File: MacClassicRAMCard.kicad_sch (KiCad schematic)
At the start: 22 parts, among them J1 RAM Exp., U1 AS4C1M16F5, U2 AS4C1M16F5, U3 74HCT08D

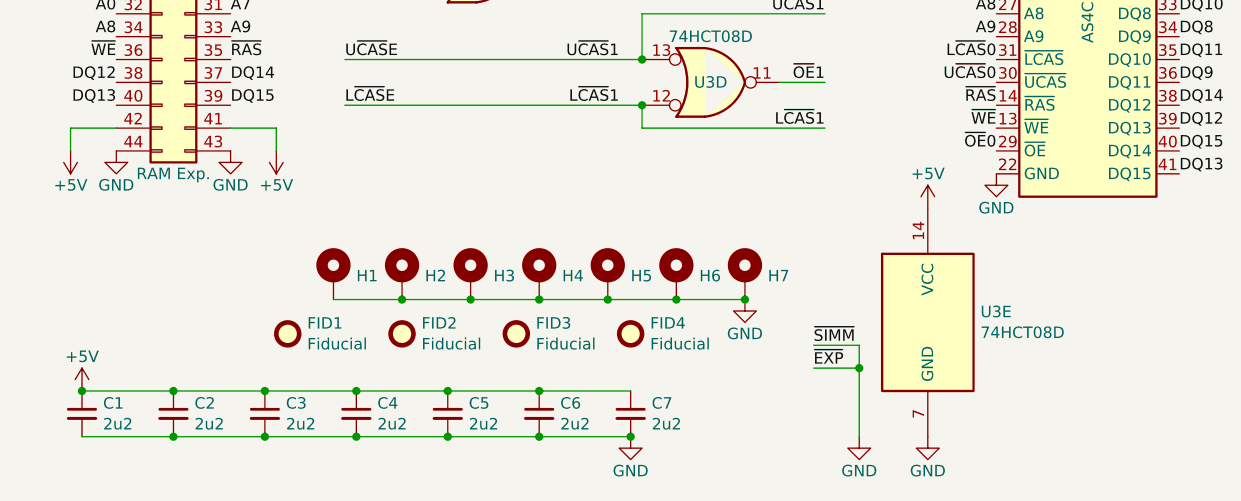
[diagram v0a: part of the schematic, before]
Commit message: New logo
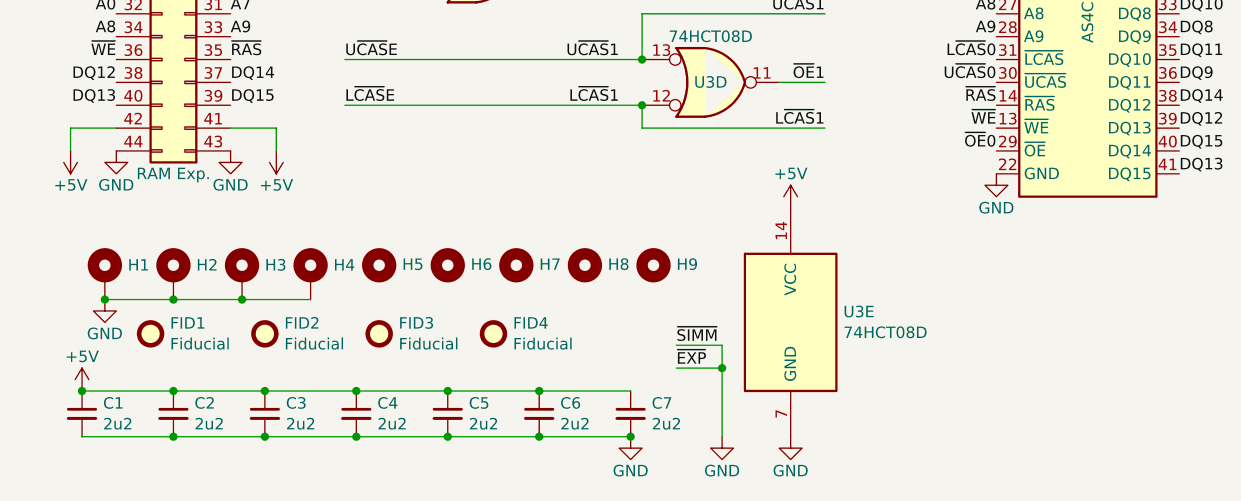
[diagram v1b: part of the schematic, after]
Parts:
- added H8, H9: (no value), stdpads:PasteHole_3mm_NPTH, symbol Mechanical:MountingHole
- H5, H6, H7: symbol Mechanical:MountingHole_Pad -> Mechanical:MountingHole
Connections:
- net GND: no longer H5.1, H6.1, H7.1
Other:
- moved on the sheet: FID1, FID2, FID3, FID4, H1, H2, H3, H4, U3E
